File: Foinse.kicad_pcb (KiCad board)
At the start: 2 copper layers, 100 x 100 mm, 124 parts, among them J1 Conn_ARM_JTAG_SWD_10, J10 Conn_02x03_Odd_Even, J3 ESQ-110-14-G-D, J4 2060-1452/998-404, J8 2601-1108, J9 USB_C_Receptacle_USB2.0_16P, Q1 AO3400A, Q10 AO3400A, Q11 AO3400A, Q12 AO3400A, Q2 AO3400A, Q3 AO3400A, Q4 AO3400A, Q5 AO3400A, Q6 AO3400A, Q7 AO3400A, Q8 AO3400A, Q9 AO3400A, U1 STM32F072C8Tx, U10 LTV-817, U11 LTV-817, U12 LTV-817, U13 LTV-817, U14 USBLC6-2SC6, U15 INA239AIDGSR, U3 LTV-817, U4 TJA1051T-3, U5 TPS563203, U6 TPS563203, U7 LTV-817, U8 LTV-817, U9 LTV-817

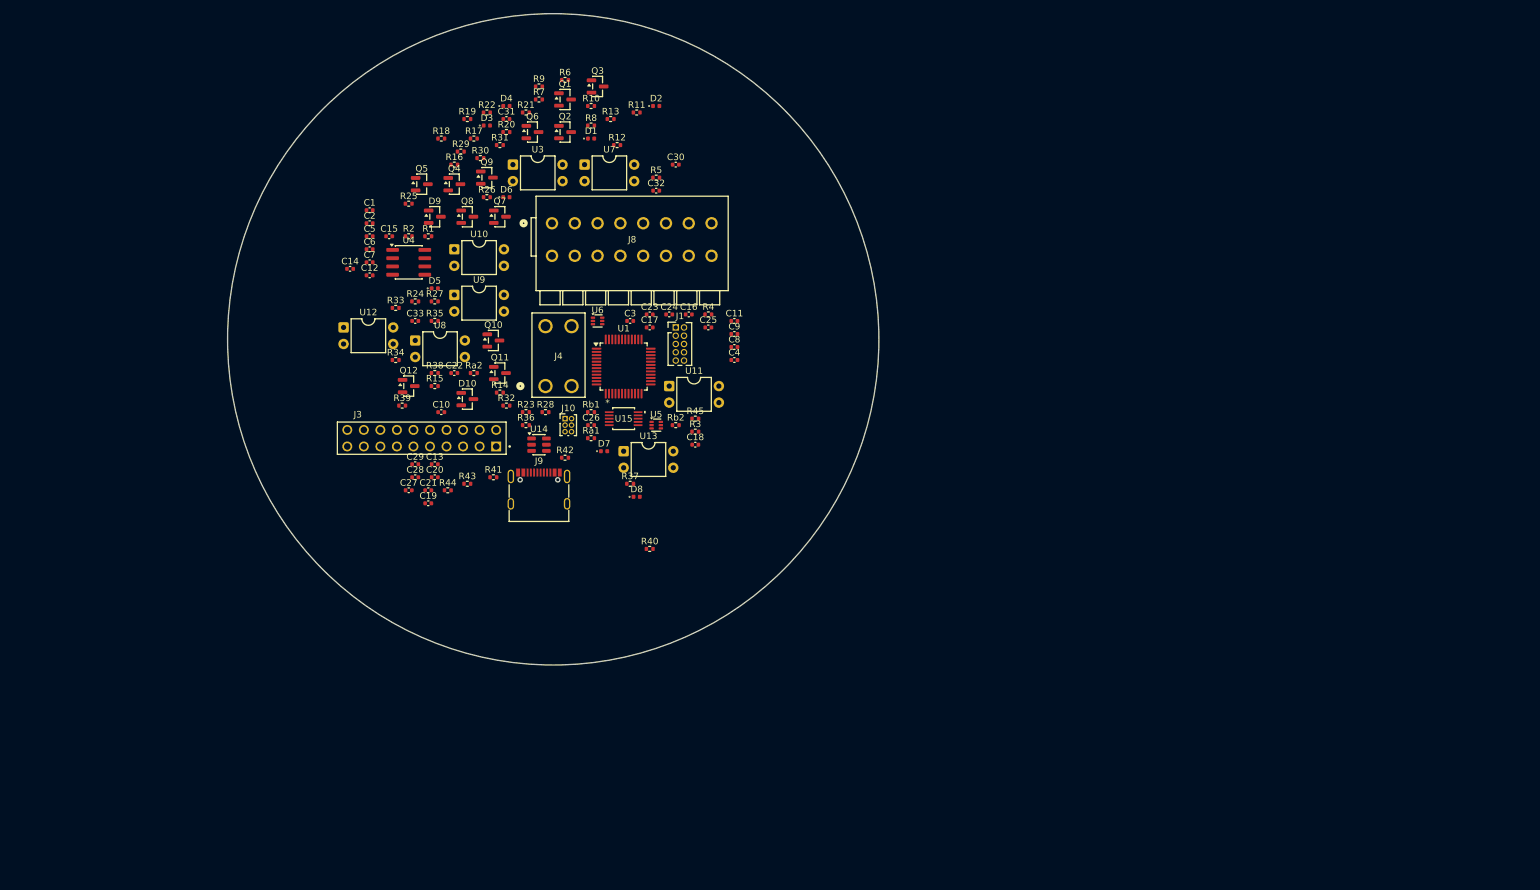
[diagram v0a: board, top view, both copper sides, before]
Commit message: Fixed shit
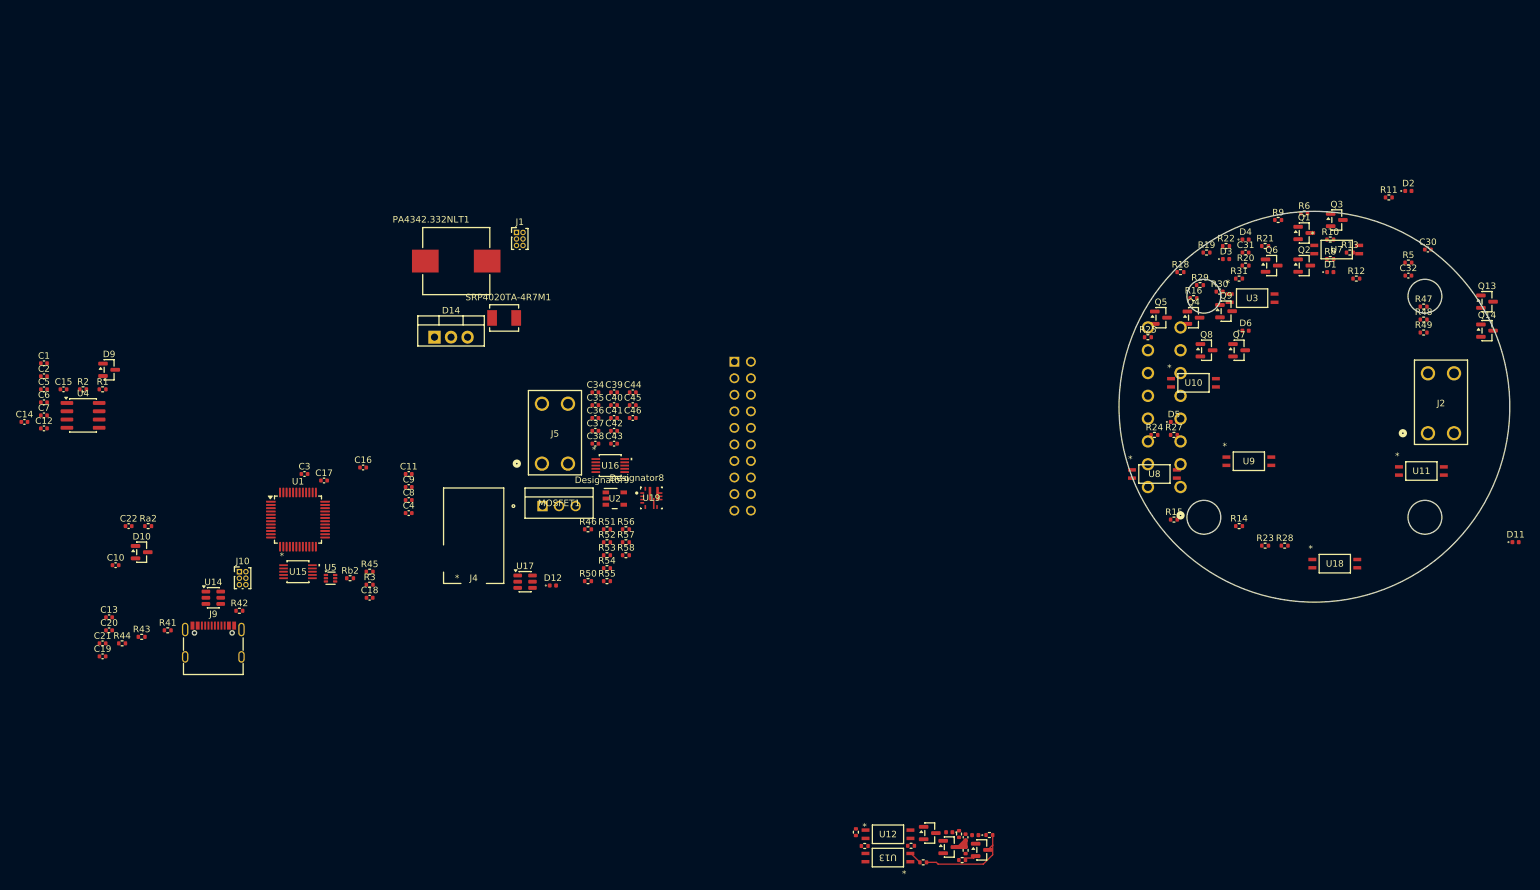
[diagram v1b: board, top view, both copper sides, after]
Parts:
- removed C23: 10 uF, Capacitor_SMD:C_0402_1005Metric
- removed C24, C25, C29: 100 nF, Capacitor_SMD:C_0402_1005Metric
- removed C26: 18 pF, Capacitor_SMD:C_0402_1005Metric
- removed C27, C28: 22 uF, Capacitor_SMD:C_0402_1005Metric
- removed R17, R26, R35, R7: 1-3Ω, Resistor_SMD:R_0402_1005Metric
- removed R4: 100k Ω, Resistor_SMD:R_0402_1005Metric
- removed Ra1: 220 Ω, Resistor_SMD:R_0402_1005Metric
- removed Rb1: 30 Ω, Resistor_SMD:R_0402_1005Metric
- removed U6: TPS563203, Package_TO_SOT_SMD:SOT-563
- added C34: 100nF, Capacitor_SMD:C_0402_1005Metric, F.Cu at (134.7, 88.0)
- added C35: 100nF, Capacitor_SMD:C_0402_1005Metric, F.Cu at (134.7, 89.9)
- added C36: 47 nF, Capacitor_SMD:C_0402_1005Metric, F.Cu at (134.7, 91.9)
- added C37: 0.1 uF, Capacitor_SMD:C_0402_1005Metric, F.Cu at (134.7, 93.9)
- added C38: 10 uF, Capacitor_SMD:C_0402_1005Metric, F.Cu at (134.7, 95.8)
- added C39: 10 uF, Capacitor_SMD:C_0402_1005Metric, F.Cu at (137.5, 88.0)
- added C40: 0.1 uF, Capacitor_SMD:C_0402_1005Metric, F.Cu at (137.5, 89.9)
- added C41: 150 pF, Capacitor_SMD:C_0402_1005Metric, F.Cu at (137.5, 91.9)
- added C42: 22 uF, Capacitor_SMD:C_0402_1005Metric, F.Cu at (137.5, 93.9)
- added C43: 22 uF, Capacitor_SMD:C_0402_1005Metric, F.Cu at (137.5, 95.8)
- added C44: 22 uF, Capacitor_SMD:C_0402_1005Metric, F.Cu at (140.4, 88.0)
- added C45: 22 uF, Capacitor_SMD:C_0402_1005Metric, F.Cu at (140.4, 89.9)
- added C46: 22 uF, Capacitor_SMD:C_0402_1005Metric, F.Cu at (140.4, 91.9)
- added D11: RED LED, LED_SMD:LED_0402_1005Metric, F.Cu at (275.9, 111.0)
- added D12: RED LED, LED_SMD:LED_0402_1005Metric, F.Cu at (128.1, 117.6)
- added D14: D_Schottky, Package_TO_SOT_THT:TO-220-3_Vertical, F.Cu at (110.0, 79.5)
- added J2: 2060-1452, Foinse Footprints:WAG, F.Cu at (262.5, 94.2)
- added J5: 2060-1452/998-404, Foinse Footprints:WAG, F.Cu at (126.5, 98.9)
- added MOSFET1: IPP80P03P4L04AKSA1, Foinse Footprints:IPP80P03P4L04AKSA1, F.Cu at (126.5, 105.4)
- added PA4342.332NLT1: 3.3 uH, Foinse Footprints:IND_PA4342.332NLT, F.Cu at (113.3, 67.8)
- added Q13: AO3400A, Package_TO_SOT_SMD:SOT-23, F.Cu at (271.6, 74.0)
- added Q14: AO3400A, Package_TO_SOT_SMD:SOT-23, F.Cu at (271.6, 78.5)
- added R46: 10 mΩ, Resistor_SMD:R_0402_1005Metric, F.Cu at (133.5, 109.0)
- added R47: 220 Ω, Resistor_SMD:R_0402_1005Metric, F.Cu at (261.8, 74.8)
- added R48: 10k Ω, Resistor_SMD:R_0402_1005Metric, F.Cu at (261.8, 76.8)
- added R49: 4.7k Ω, Resistor_SMD:R_0402_1005Metric, F.Cu at (261.8, 78.8)
- added R50: 3.3k Ω, Resistor_SMD:R_0402_1005Metric, F.Cu at (133.5, 117.0)
- added R51: 52.3k Ω, Resistor_SMD:R_0402_1005Metric, F.Cu at (136.4, 109.0)
- added R52: 169k Ω, Resistor_SMD:R_0402_1005Metric, F.Cu at (136.4, 111.0)
- added R53: 36.1k Ω, Resistor_SMD:R_0402_1005Metric, F.Cu at (136.4, 113.0)
- added R54: DNP, Resistor_SMD:R_0402_1005Metric, F.Cu at (136.4, 115.0)
- added R55: 49.9 Ω, Resistor_SMD:R_0402_1005Metric, F.Cu at (136.4, 117.0)
- added R56: 73.2 Ω, Resistor_SMD:R_0402_1005Metric, F.Cu at (139.3, 109.0)
- added R57: DNP, Resistor_SMD:R_0402_1005Metric, F.Cu at (139.3, 111.0)
- added R58: 10k Ω, Resistor_SMD:R_0402_1005Metric, F.Cu at (139.3, 113.0)
- added SRP4020TA-4R7M1: 4.7 uH, Foinse Footprints:IND_SRP4020TA-4R7M, F.Cu at (120.7, 76.5)
- added U16: INA239AIDGSR, Foinse Footprints:VSSOP_9AIDGST_TEX, F.Cu at (136.9, 99.2)
- added U17: LTC4412xS6, Package_TO_SOT_SMD:TSOT-23-6, F.Cu at (123.9, 117.0)
- added U18: LTV-817, Foinse Footprints:SO4_TOS, F.Cu at (248.2, 114.3)
- added U19: TPS56A37RPAR, Foinse Footprints:RPA0010A-MFG, F.Cu at (143.3, 104.2)
- added U2: TLV70433DBVT, Foinse Footprints:DBV0005A_N, F.Cu at (137.6, 104.3)
- C17: value 100 nF -> 0.1 uF
- J1: value Conn_ARM_JTAG_SWD_10 -> Conn_02x03_Odd_Even; footprint Connector_PinHeader_1.27mm:PinHeader_2x05_P1.27mm_Vertical -> Connector_PinHeader_1.00mm:PinHeader_2x03_P1.00mm_Vertical
- J3, J8: moved to B.Cu
- J4: value 2060-1452/998-404 -> PJ-002AH; footprint Foinse Footprints:WAG -> Foinse Footprints:PJ-002AH_CUD
- R10, R30, R39: value 2 Ω -> 2 kΩ
- R11, R40: value 4.7 Ω -> 4.7 kΩ
- R20: value 6 Ω -> 6k Ω
- R21: value 2 Ω -> 2k Ω
- R22, R31: value 4.7 Ω -> 4.7k Ω
- R29, R38, R9: value 6 Ω -> 6 kΩ
- U10, U11, U12, U13, U3, U7, U8, U9: footprint Package_DIP:DIP-4_W7.62mm -> Foinse Footprints:SO4_TOS
- moved U9 124.6 mm to (235.0, 98.5)
- moved C30 116.2 mm to (262.5, 66.0)
- moved C32 116.2 mm to (259.5, 70.0)
- moved D2 116.2 mm to (259.5, 57.0)
- moved R11 116.2 mm to (256.5, 58.0)
- moved R5 116.2 mm to (259.5, 68.0)
- moved U11 116.2 mm to (261.5, 100.0)
- moved U7 116.2 mm to (248.5, 66.0)
- moved C33 115.9 mm to (191.5, 156.3), turned to -90 degrees
- moved C31 115.3 mm to (234.5, 66.5)
- moved D1 115.3 mm to (247.5, 69.5)
- moved D3 115.3 mm to (231.5, 67.5)
- moved D4 115.3 mm to (234.5, 64.5)
- moved D5 115.3 mm to (223.5, 92.5)
- moved D6 115.3 mm to (234.5, 78.5)
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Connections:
- C30 pad 1: VBAT_DROGUE -> VBAT_AUX1
- C31 pad 1: VBAT_MAIN -> VBAT_AUX1
- C33 pad 1: VBAT_AUX2 -> VBAT_AUX1
- D1 pad 2: VBAT_DROGUE -> VBAT_AUX1
- D2 pad 2: VBAT_DROGUE -> VBAT_AUX1
- D3 pad 2: VBAT_MAIN -> VBAT_AUX1
- D4 pad 2: VBAT_MAIN -> VBAT_AUX1
- D7 pad 2: VBAT_AUX2 -> VBAT_AUX1
- D8 pad 2: VBAT_AUX2 -> VBAT_AUX1
- D9 pad 1: CAN_hi -> CAN_BUS+
- D9 pad 2: CAN_lo -> CAN_BUS+-
- J1 pad 1: 3.3V -> NRST
- J1 pad 6: unconnected-(J1-SWO/TDO-Pad6) -> 3.3V
- J10 pad 3: PA- -> PA_-
- J8 pad 1: VBAT_DROGUE -> VBAT_AUX1
- J8 pad 13: VBAT_AUX2 -> VBAT_AUX1
- J8 pad 14: VBAT_AUX2 -> VBAT_AUX1
- J8 pad 2: VBAT_DROGUE -> VBAT_AUX1
- J8 pad 5: VBAT_MAIN -> VBAT_AUX1
- J8 pad 6: VBAT_MAIN -> VBAT_AUX1
- Q1 pad 3: Net-(Q1-D) -> /Drogue neg
- Q10 pad 3: Net-(Q10-D) -> /Aux2 neg
- Q4 pad 3: Net-(Q4-D) -> /Main neg
- Q7 pad 3: Net-(Q7-D) -> /Aux1 neg
- R1 pad 2: CAN_lo -> CAN_BUS+-
- R12 pad 1: PGND -> GND
- R14 pad 1: PGND -> GND
- R2 pad 1: CAN_hi -> CAN_BUS+
- R23 pad 1: PGND -> GND
- R32 pad 1: PGND -> GND
- R45 pad 1: VBAT -> VBAT_BS
- R45 pad 2: Net-(U15-IN-) -> VBAT
- U1 pad 28: unconnected-(U1-PB15-Pad28) -> SERVO_CURRENT_CS
- U1 pad 43: unconnected-(U1-PB7-Pad43) -> PYRO_ON
- U1 pad 45: unconnected-(U1-PB8-Pad45) -> Mode_sel
- U10 pad 2: PGND -> GND
- U12 pad 2: PGND -> GND
- U12 pad 4: VBAT_AUX2 -> VBAT_AUX1
- U13 pad 1: VBAT_AUX2 -> VBAT_AUX1
- U14 pad 3: USB_D_ -> USB_D-
- U15 pad 10: VBAT -> VBAT_BS
- U15 pad 8: VBAT -> VBAT_BS
- U15 pad 9: Net-(U15-IN-) -> VBAT
- U3 pad 2: PGND -> GND
- U3 pad 4: VBAT_DROGUE -> VBAT_AUX1
- U4 pad 6: CAN_lo -> CAN_BUS+-
- U4 pad 7: CAN_hi -> CAN_BUS+
- U7 pad 1: VBAT_DROGUE -> VBAT_AUX1
- U8 pad 2: PGND -> GND
- U8 pad 4: VBAT_MAIN -> VBAT_AUX1
- U9 pad 1: VBAT_MAIN -> VBAT_AUX1
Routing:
- net Net-(Q12-D): track 0.00 -> 14.9 mm
- net /Aux2 neg: track 0.00 -> 4.58 mm
- net Net-(R37-Pad1): track 0.00 -> 2.04 mm
- net PGND: track 0.00 -> 1.94 mm
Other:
- board size 100 x 100 mm -> 60 x 60 mm
- copper layers 2 -> 4
- board text added: "*"
